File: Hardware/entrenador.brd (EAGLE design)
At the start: 121.9 x 70.8 mm, 68 parts, among them U1 DRV8833

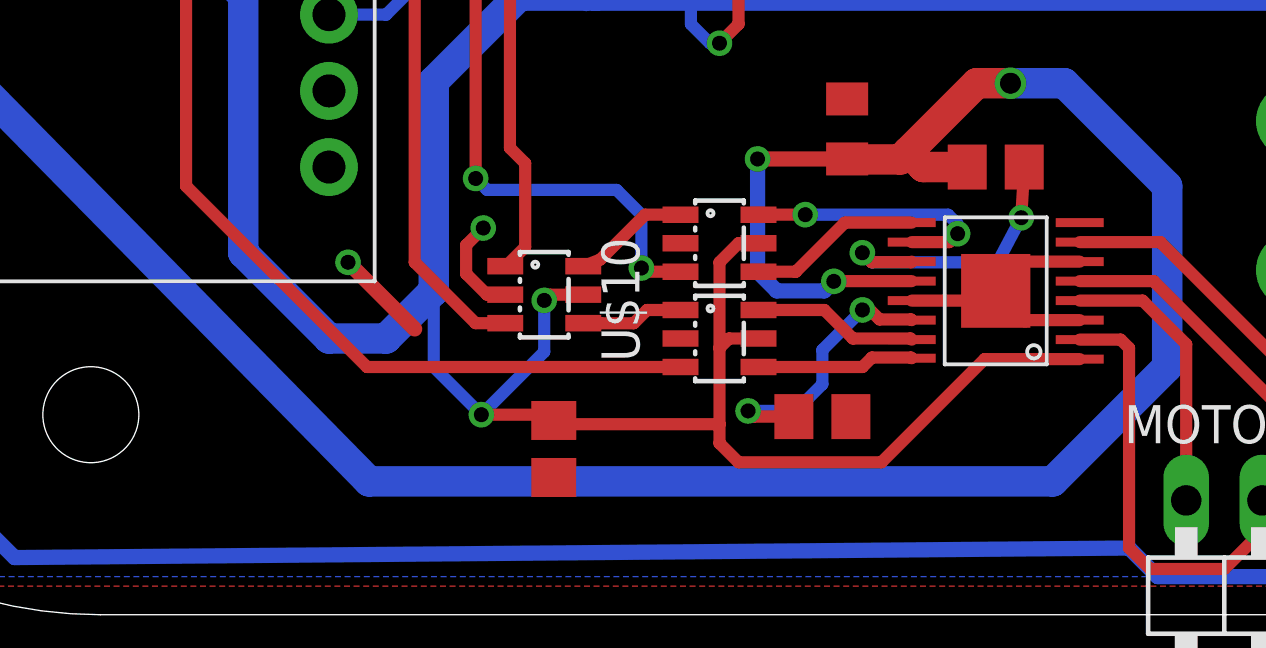
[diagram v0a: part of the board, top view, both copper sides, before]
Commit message: me falto revisar una cosa del anterior commit, disculpas. curregido
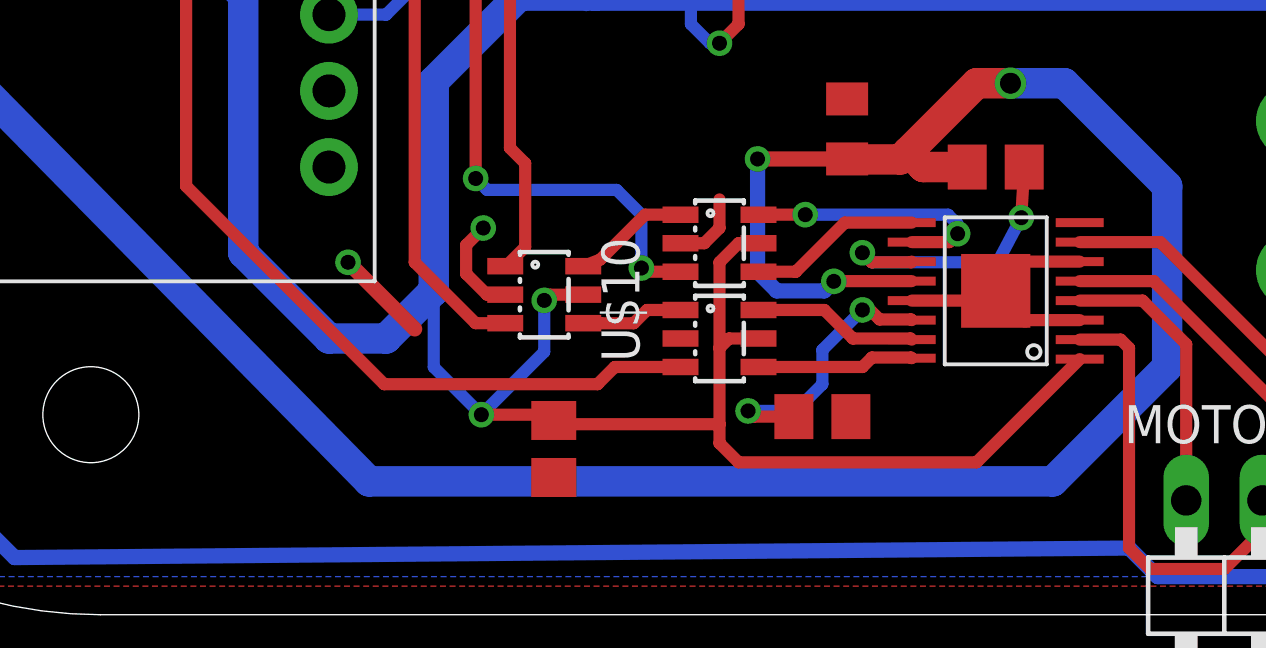
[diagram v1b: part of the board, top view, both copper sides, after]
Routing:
- net GND: track 15.8 -> 18.3 mm
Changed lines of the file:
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@@
 <contactref element="C15" pad="2"/>
 <contactref element="C16" pad="2"/>
-<wire x1="34.26" y1="15.5575" x2="34.26" y2="18.7325" width="0" layer="19" extent="1-1"/>
-<wire x1="39.939" y1="12.954" x2="41.9675" y2="16.82" width="0" layer="19" extent="1-1"/>
+<wire x1="34.26" y1="18.7325" x2="35.052" y2="18.7325" width="0.4064" layer="1"/>
+<wire x1="35.052" y1="18.7325" x2="35.56" y2="19.2405" width="0.4064" layer="1"/>
+<wire x1="35.56" y1="19.2405" x2="35.56" y2="20.193" width="0.4064" layer="1"/>
 </signal>
 <signal name="VCC">
@@
 <contactref element="U1" pad="1"/>
 <contactref element="C9" pad="1"/>
-<wire x1="47.5675" y1="14.87" x2="44.3975" y2="14.87" width="0.4064" layer="1"/>
-<wire x1="44.3975" y1="14.87" x2="40.9575" y2="11.43" width="0.4064" layer="1"/>
-<wire x1="40.9575" y1="11.43" x2="36.195" y2="11.43" width="0.4064" layer="1"/>
+<wire x1="44.1275" y1="11.43" x2="36.195" y2="11.43" width="0.4064" layer="1"/>
 <wire x1="36.195" y1="11.43" x2="35.56" y2="12.065" width="0.4064" layer="1"/>
 <wire x1="35.56" y1="12.065" x2="35.56" y2="12.7" width="0.4064" layer="1"/>
@@
 <wire x1="29.718" y1="16.8275" x2="29.718" y2="15.113" width="0.4064" layer="16"/>
 <wire x1="29.718" y1="15.113" x2="27.6225" y2="13.0175" width="0.4064" layer="16"/>
+<wire x1="44.1275" y1="11.43" x2="47.5675" y2="14.87" width="0.4064" layer="1"/>
 </signal>
 <signal name="M1B">
@@
 <contactref element="U$8" pad="P$5"/>
 <contactref element="U$1" pad="3"/>
-<wire x1="23.81" y1="14.6075" x2="17.78" y2="20.6375" width="0.4064" layer="1"/>
 <wire x1="17.78" y1="20.6375" x2="17.78" y2="38.1" width="0.4064" layer="1"/>
 <via x="17.78" y="38.1" extent="1-16" drill="0.5"/>
@@
 <wire x1="20.0025" y1="51.1175" x2="20.6375" y2="51.7525" width="0.4064" layer="16"/>
 <wire x1="20.6375" y1="51.7525" x2="22.5425" y2="51.7525" width="0.4064" layer="16"/>
-<wire x1="34.26" y1="14.6075" x2="23.81" y2="14.6075" width="0.4064" layer="1"/>
+<wire x1="34.26" y1="14.6075" x2="32.07" y2="14.6075" width="0.4064" layer="1"/>
+<wire x1="32.07" y1="14.6075" x2="31.496" y2="14.0335" width="0.4064" layer="1"/>
+<wire x1="31.496" y1="14.0335" x2="24.384" y2="14.0335" width="0.4064" layer="1"/>
+<wire x1="24.384" y1="14.0335" x2="17.78" y2="20.6375" width="0.4064" layer="1"/>
 </signal>
 <signal name="VIN">
